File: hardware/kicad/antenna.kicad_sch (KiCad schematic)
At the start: 13 parts, among them J6 BWIPX-1-001E

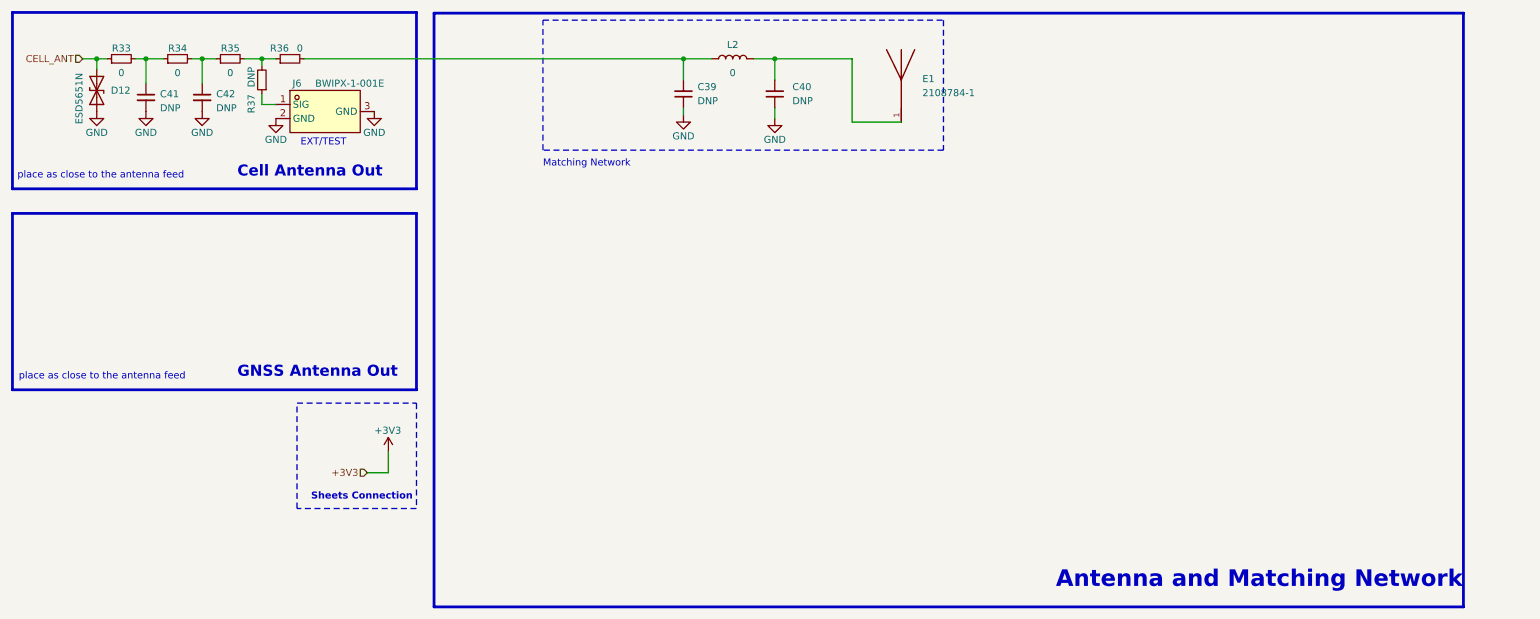
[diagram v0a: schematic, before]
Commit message: Finish Manufacturing File
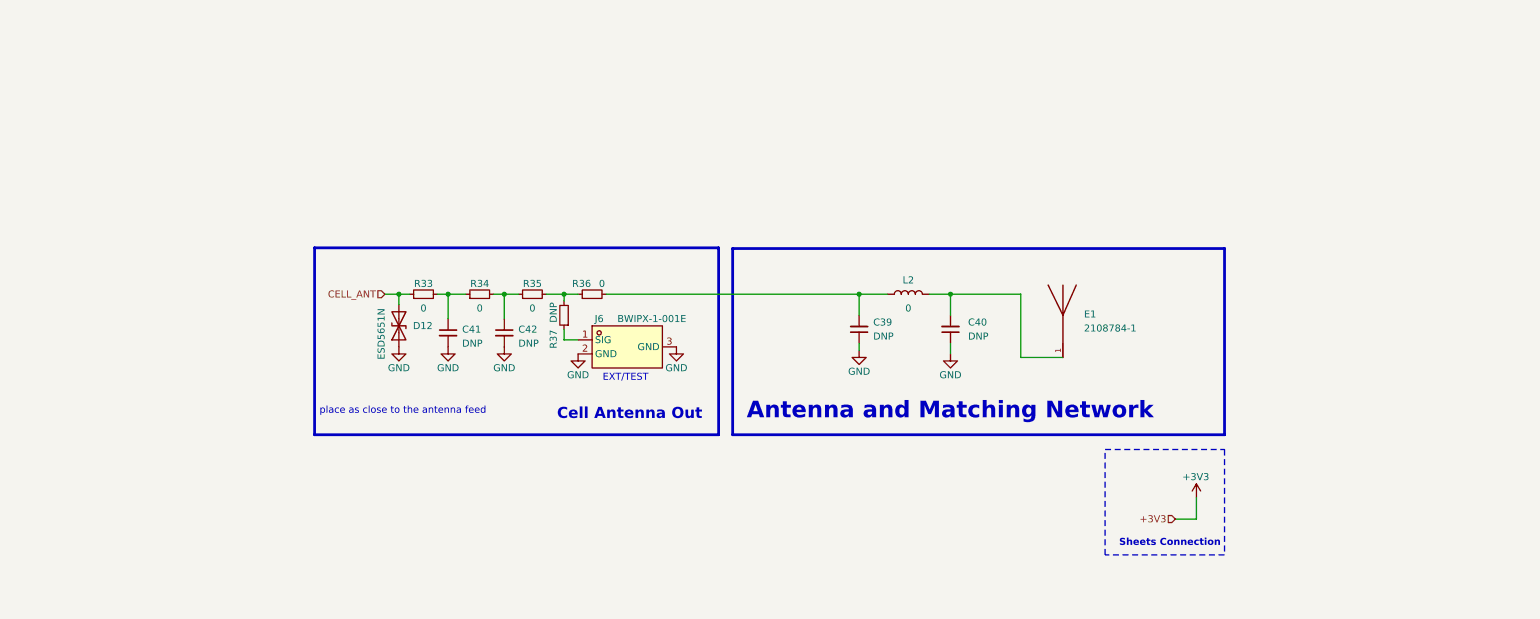
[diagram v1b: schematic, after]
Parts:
- C39: Distributor LCSC -> -; Distributor Link https://www.lcsc.com/product-detail/Multilayer-Ceramic-Capa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 -> -; Distributor Part Number C88885 -> -; Manufacturer Murata Electronics -> -; Manufacturer Part Number GJM1555C1H2R0WB01D -> -
- C40: Distributor LCSC -> -; Distributor Link https://www.lcsc.com/product-detail/Multilayer-Ceramic-Capa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 -> -; Distributor Part Number C76899 -> -; Manufacturer Murata Electronics -> -; Manufacturer Part Number GJM1555C1H1R2WB01D -> -
- C41, C42: Distributor (none) -> -; Distributor Link (none) -> -; Distributor Part Number (none) -> -; Manufacturer (none) -> -; Manufacturer Part Number (none) -> -
- E1: Distributor (none) -> TE Connectivity; Distributor Link (none) -> https://www.te.com/en/product-2108784-1.html; Distributor Part Number (none) -> -; Manufacturer (none) -> TE Connectivity; Manufacturer Part Number (none) -> 2108784-1
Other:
- note removed: "GNSS Antenna Out"
- note removed: "Matching Network"
- moved on the sheet: C39, C40, C41, C42, D12, E1, J6, L2, R33, R34, R35, R36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
